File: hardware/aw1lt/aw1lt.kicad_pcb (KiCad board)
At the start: 2 copper layers, 30 x 22 mm, 27 parts, among them J1 ISP_FTDI, Q1 BSS138, SW1 SW_Push, SW2 SW_Push, SW3 SW_Push, U1 DS3231MZ, U2 ATMEGA328P-AU

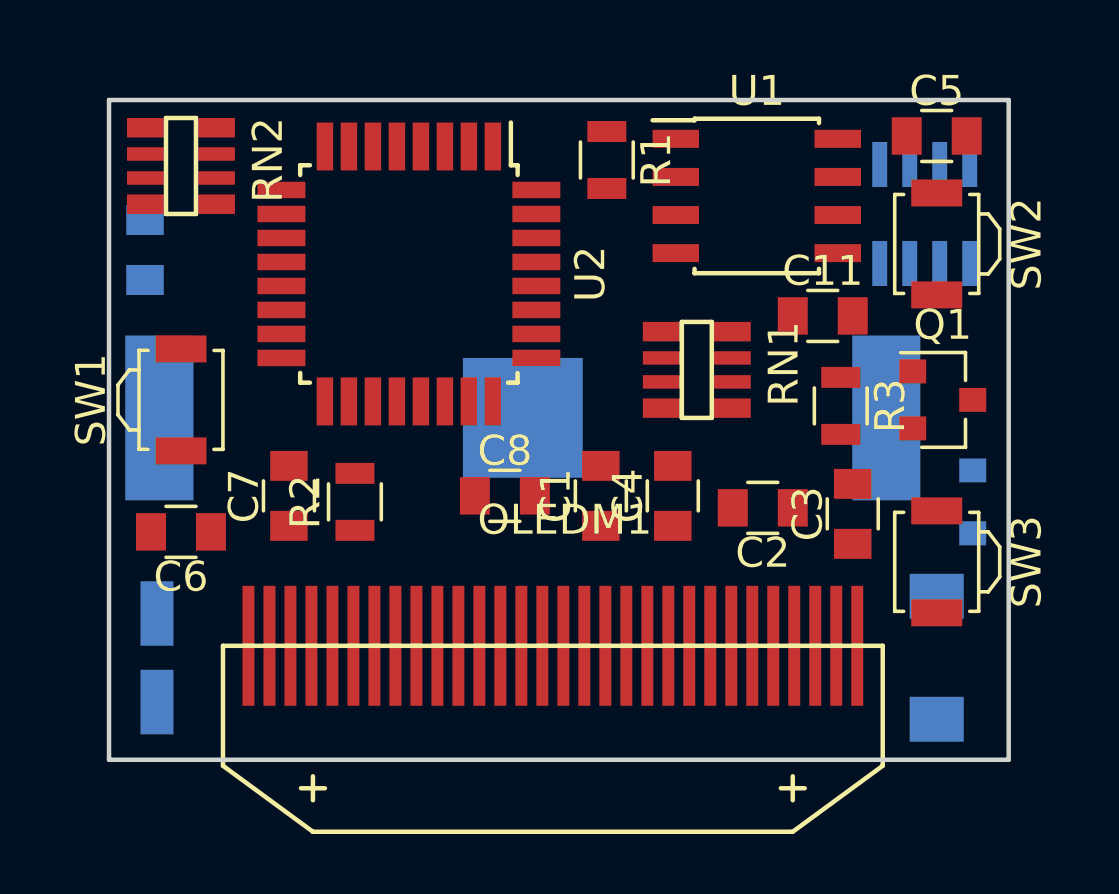
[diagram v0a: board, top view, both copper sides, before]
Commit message: starting to set tracks down
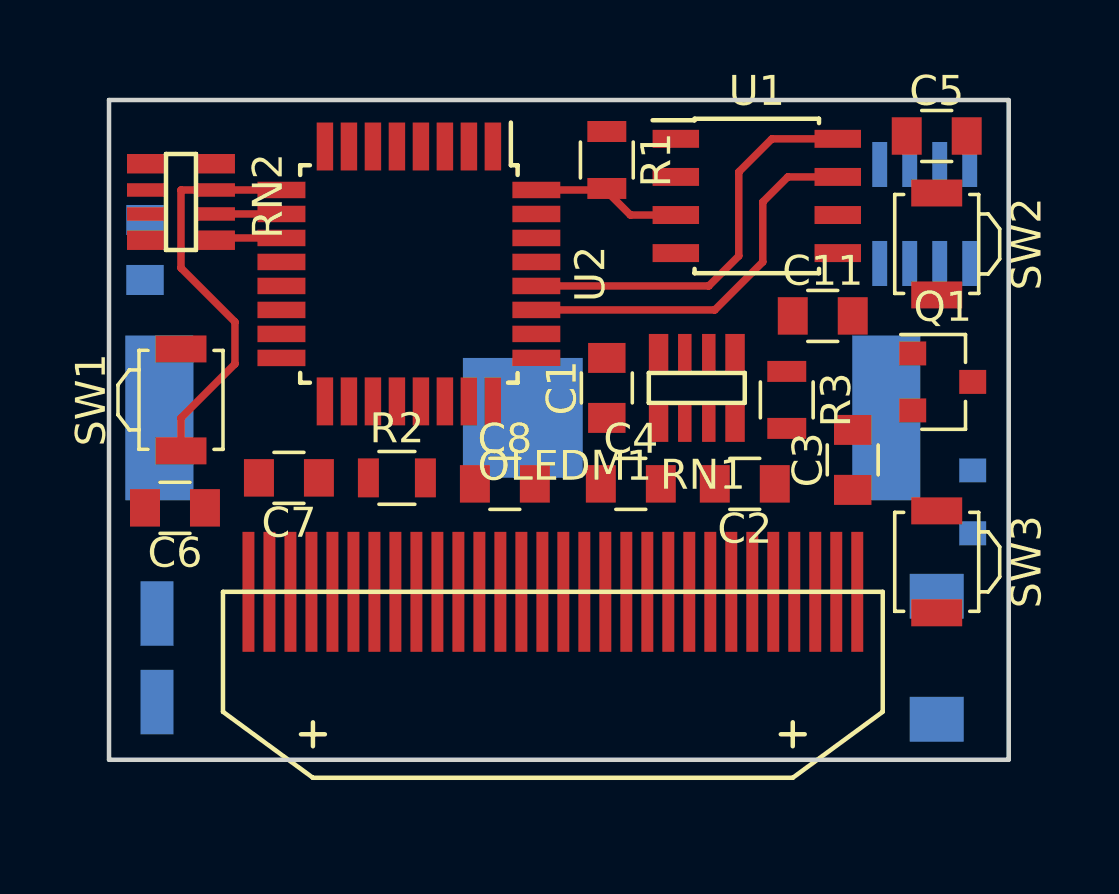
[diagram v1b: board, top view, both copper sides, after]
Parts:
- Q1: value BSS138 -> Q_NPN_CBE
- moved C1 3.61 mm to (141.6, 134.6)
- moved R3 1.81 mm to (147.6, 135.0)
- moved C3 1.80 mm to (149.8, 137.0)
- moved OLEDM1 1.80 mm to (139.8, 141.4)
- moved R2 1.61 mm to (134.6, 137.6), turned to 0 degrees
- moved C4 1.46 mm to (142.4, 137.8), turned to 0 degrees
- moved RN2 1.20 mm to (127.4, 128.4)
- moved C2 1.00 mm to (146.2, 137.8)
- moved C6 0.82 mm to (127.2, 138.6)
- moved C7 0.60 mm to (131.0, 137.6), turned to 180 degrees
- moved Q1 0.60 mm to (152.8, 134.4)
- moved RN1 0.60 mm to (144.6, 134.6), turned to 0 degrees
- moved C8 0.40 mm to (138.2, 137.8)
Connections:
- Q1 pad 1: Net-(Q1-Pad1) -> Net-(BZ1-Pad2)
- Q1 pad 2: GND -> Net-(Q1-Pad2)
- Q1 pad 3: Net-(BZ1-Pad2) -> GND
- R3 pad 1: Net-(Q1-Pad1) -> Net-(Q1-Pad2)
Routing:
- net SCL: track 0.00 -> 13.7 mm
- net PB0: track 0.00 -> 13.5 mm
- net SDA: track 0.00 -> 13.1 mm
- net INT0: track 0.00 -> 5.00 mm
- net PB2: track 0.00 -> 2.23 mm
- net PB1: track 0.00 -> 2.20 mm

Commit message: still trying to figure out this routing and placement...
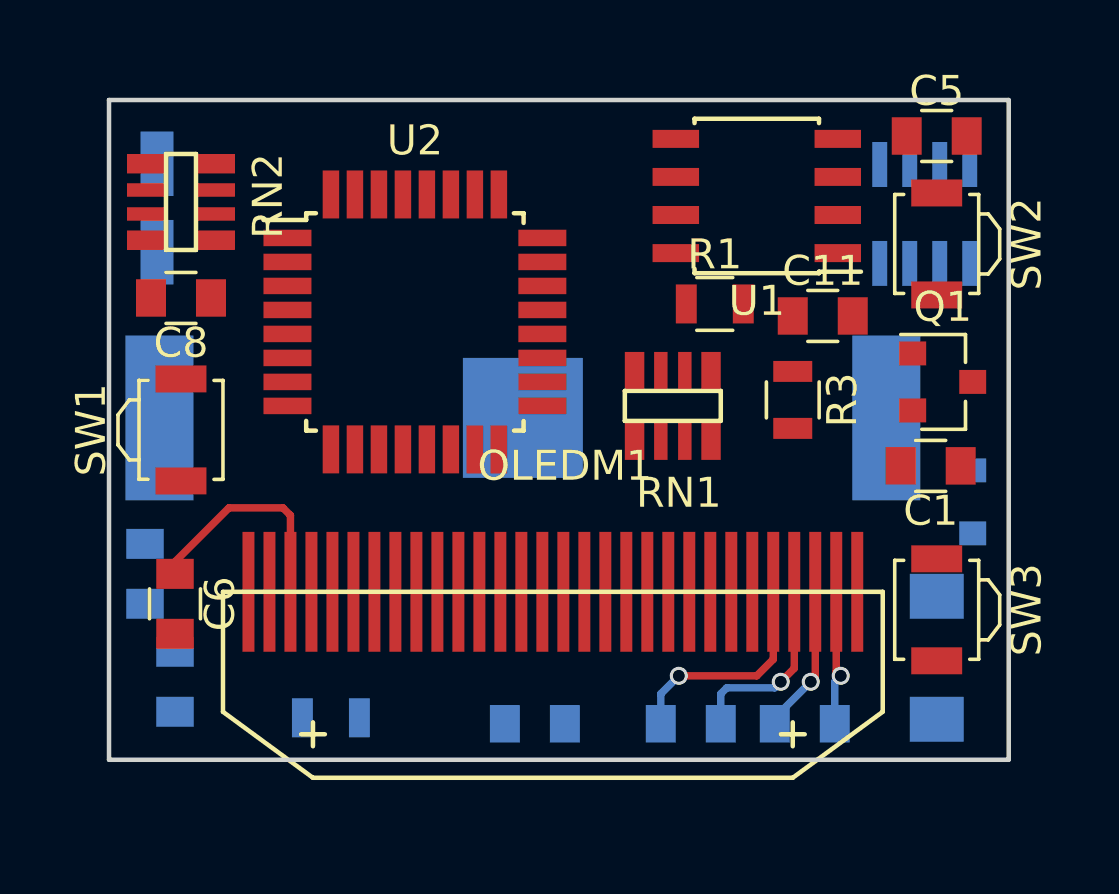
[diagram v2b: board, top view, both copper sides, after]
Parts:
- C2, C3, C4, C7, R2: moved to B.Cu
- moved C9 15.0 mm to (126.6, 128.6)
- moved C8 12.5 mm to (127.4, 131.6), turned to 180 degrees
- moved C1 11.1 mm to (152.4, 137.2), turned to 180 degrees
- moved C10 10.8 mm to (126.2, 140.8)
- moved C3 8.94 mm to (148.2, 145.8), turned to 180 degrees
- moved C4 8.62 mm to (139.2, 145.8), turned to 180 degrees
- moved R2 8.30 mm to (132.4, 145.6)
- moved C2 8.20 mm to (144.4, 145.8)
- moved C7 7.79 mm to (127.2, 144.4), turned to 90 degrees
- moved R1 6.00 mm to (145.2, 131.8), turned to 0 degrees
- moved C6 3.20 mm to (127.2, 141.8), turned to 270 degrees
- moved U2 1.61 mm to (135.2, 132.4), turned to 0 degrees
- moved SW3 1.60 mm to (152.6, 142.0)
- moved SW1 1.00 mm to (127.4, 136.0)
- moved RN1 1.00 mm to (143.8, 135.2)
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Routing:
- net SCL: track 13.7 -> 0.00 mm
- net PB0: track 13.5 -> 0.00 mm
- net SDA: track 13.1 -> 0.00 mm
- net Net-(C6-Pad1): track 0.00 -> 7.65 mm
- net Net-(C2-Pad2): track 0.00 -> 7.48 mm, vias 0 -> 1
- net Net-(C2-Pad1): track 0.00 -> 6.35 mm, vias 0 -> 1
- net INT0: track 5.00 -> 0.00 mm
- net Net-(C3-Pad2): track 0.00 -> 4.96 mm, vias 0 -> 1
- net Net-(C3-Pad1): track 0.00 -> 4.54 mm, vias 0 -> 1
- net PB1: track 2.20 -> 0.00 mm
- net PB2: track 2.23 -> 0.11 mm
